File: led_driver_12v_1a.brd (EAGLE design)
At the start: 45 x 19.4 mm, 53 parts, among them Q1 BSZ0902NSI, Q2 BSZ0902NSI, Q3 BSZ0902NSI, Q4 BSZ0902NSI, Q5 BSZ0902NSI, Q6 SSM3K2615R

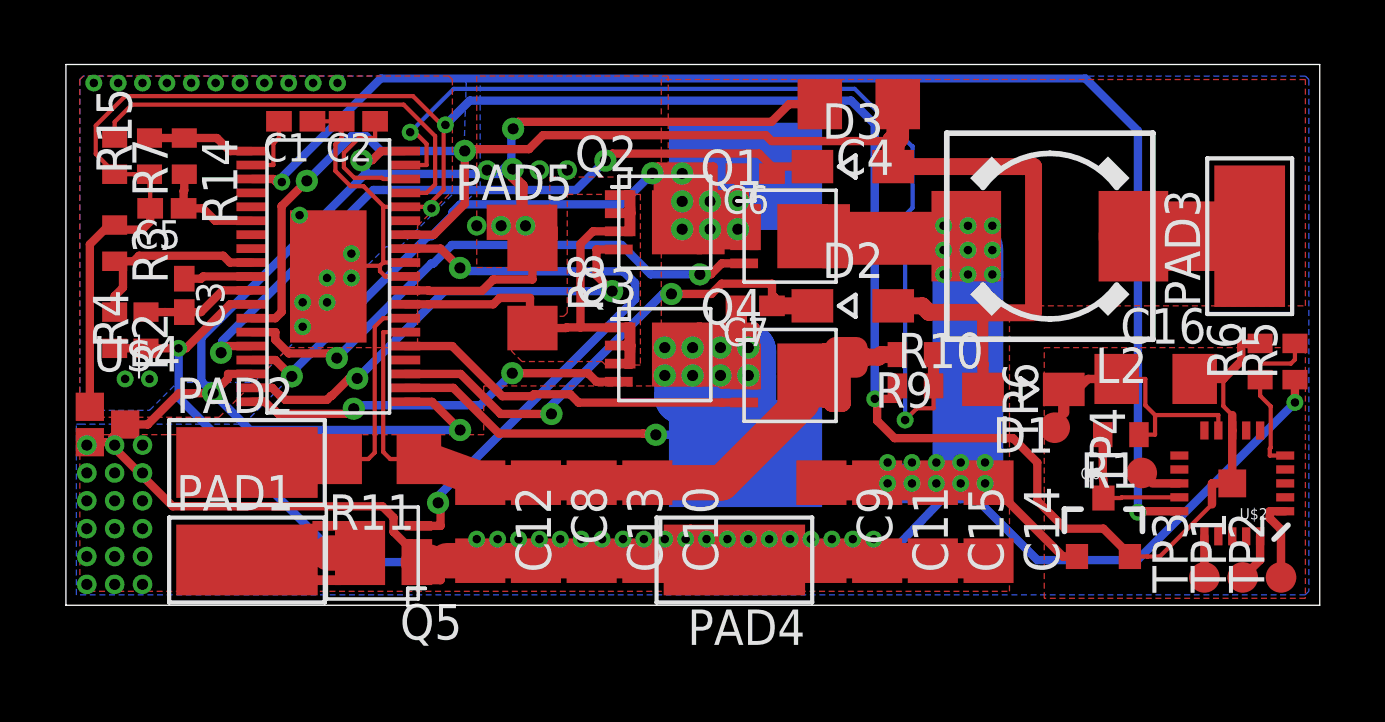
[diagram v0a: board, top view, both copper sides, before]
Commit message: Added Gerbers and PartList
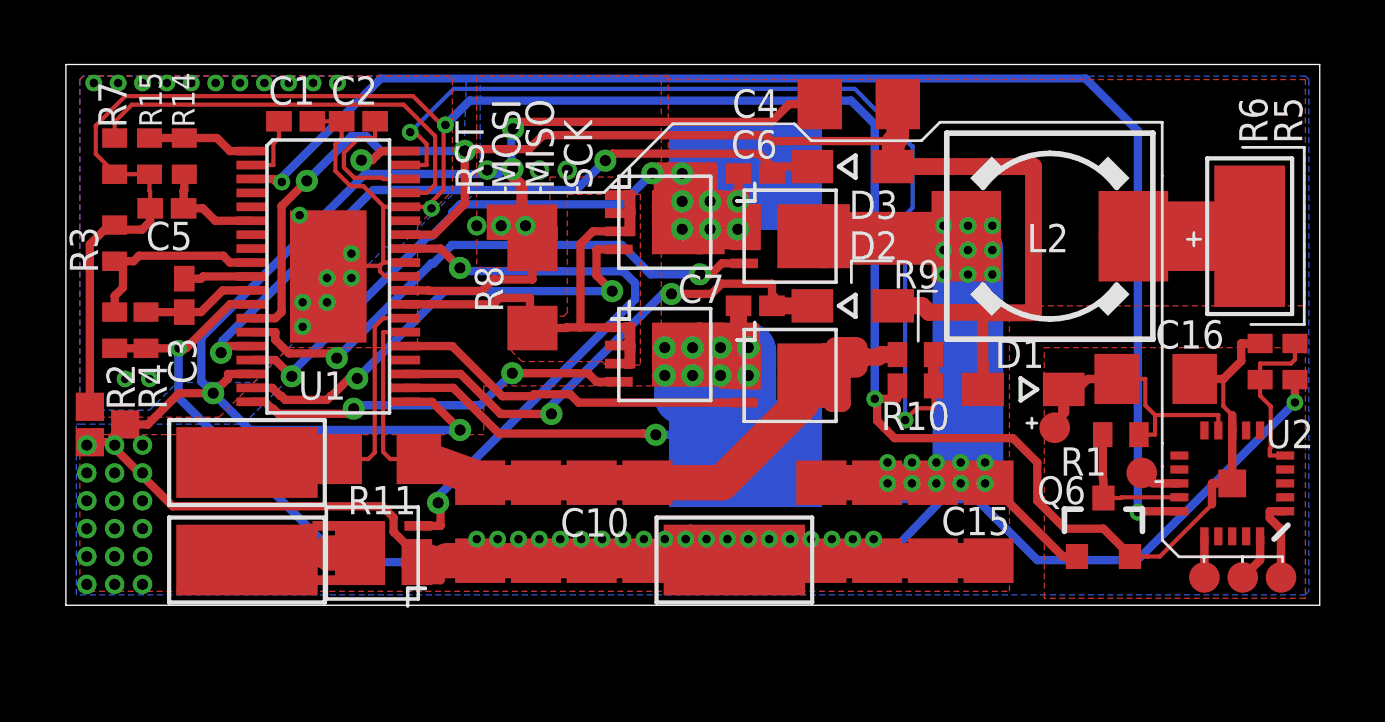
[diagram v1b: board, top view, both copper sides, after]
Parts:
- C16, C4: value 4.7uF, 25V, Low ESR (Kemet C1206C475K3RACTU) -> 4.7uF
- renumbered TP1 to MISO, TP2 to SCK, TP3 to MOSI, TP4 to RST, TP6 to VCC
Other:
- board text added: "C1,C2 22nF (0402) C3 470nF (0402) C5,C6,C7 0.1uF (0402) C4,C8-C16 4.7uF (Kemet C1206C475K3RACTU)"
- board text added: "D1"
- board text added: "D1-D3 BAT46-WJ L1 4.7u (744771004) L2 1000n (Bourns Inc. SRR7045-1R0M) Q1-Q5 BSZ0902NSI Q6 SSM3K2615R U1 LT3791 TSSOP38 U2 ATTINY24A (QFN)"
- board text added: "IN: LiPo 3S OUT: 12V/1.05A"
- board text added: "R4 50(0402) R1 10k(0402) R3,R6,R15 56.9k(0402) R7,R10 86.6k(0402) R5,R14 100k(0402) R2 300k(0402) R9 1Meg(0402) R8 10m(1206) Riedon CSR1206-0R001F1 R11 50m(1206) Ohmite MCS1632R005FER"
- board text added: "U1"
- board text added: "U2"
